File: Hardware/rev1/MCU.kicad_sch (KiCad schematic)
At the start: 5 parts, among them SW1 SW_Push, U1 STM32F103C8Tx, U4 W25Q128JVS

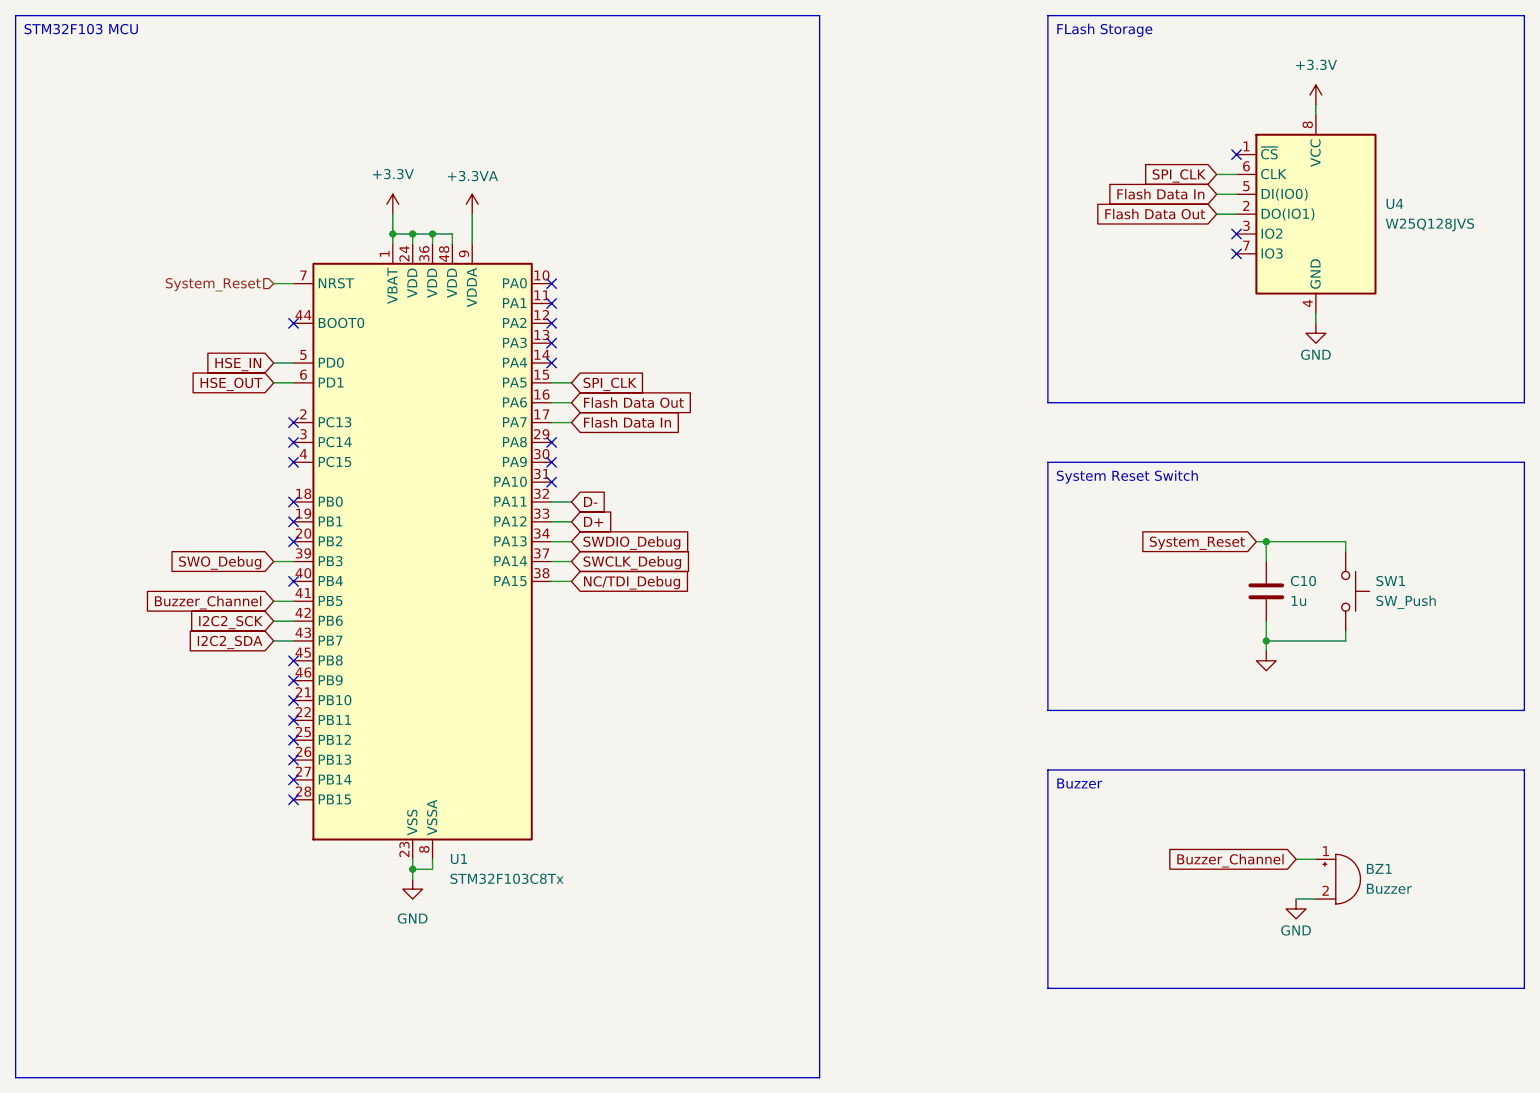
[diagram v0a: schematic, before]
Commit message: UUUUHHH
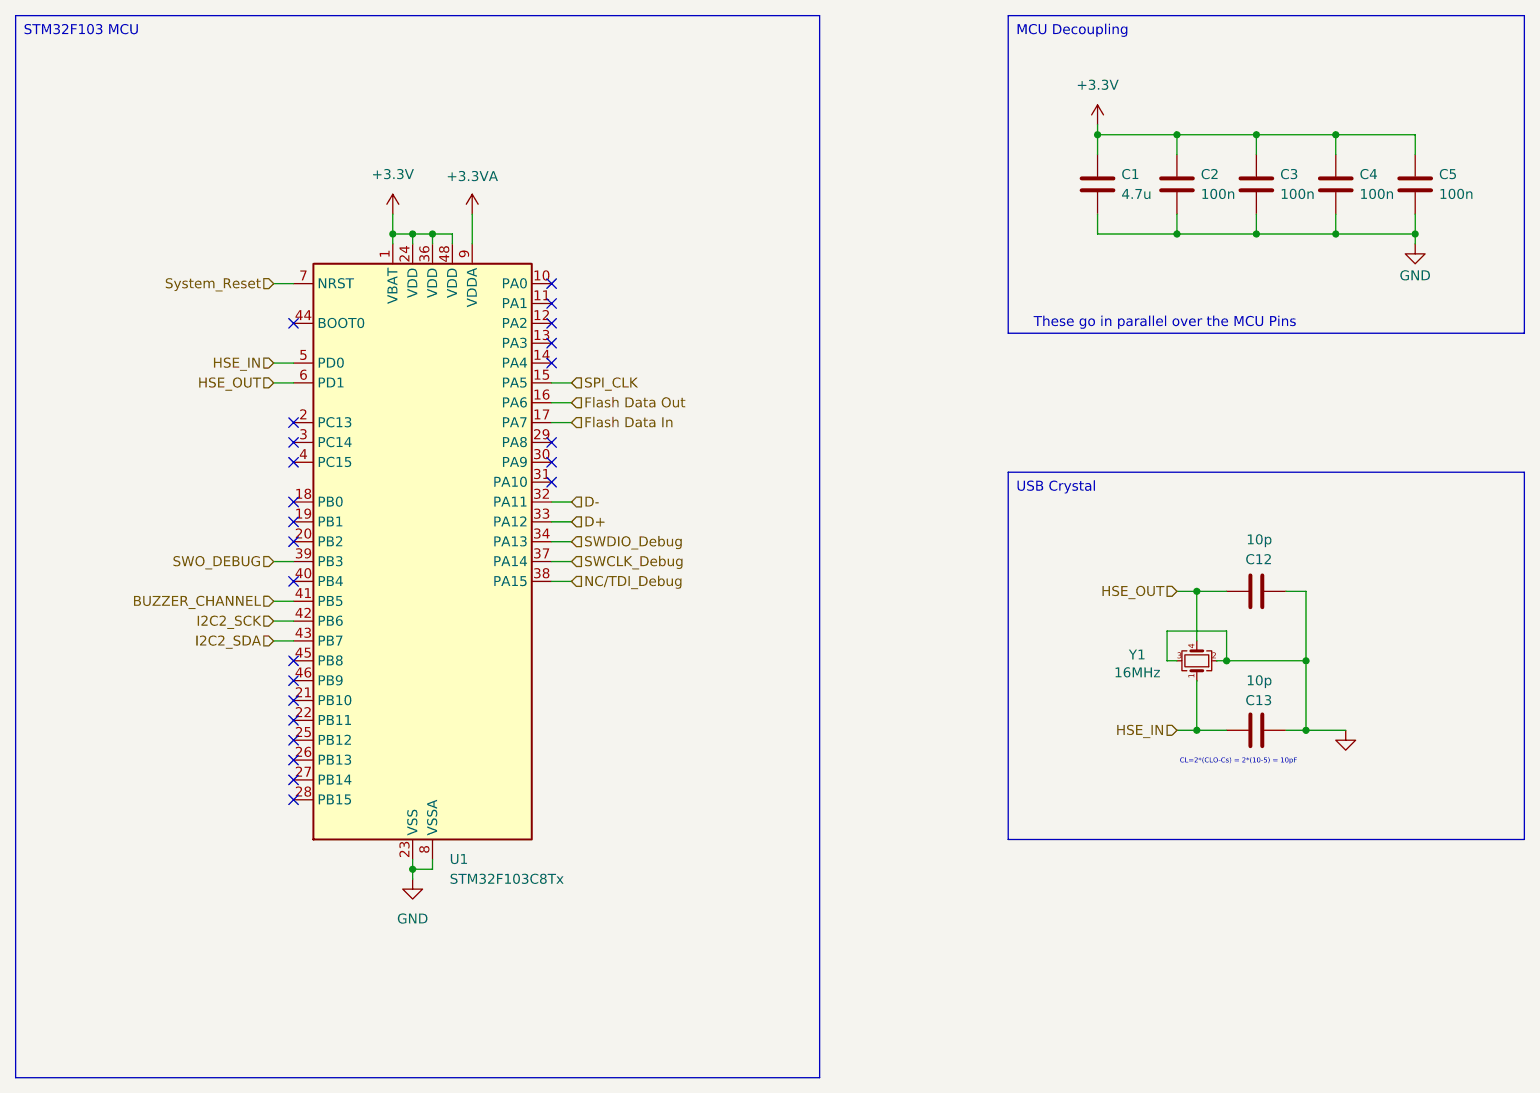
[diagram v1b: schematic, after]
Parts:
- removed BZ1: Buzzer, symbol Device:Buzzer
- removed C10: 1u, symbol Device:C
- removed SW1: SW_Push, symbol Switch:SW_Push
- removed U4: W25Q128JVS, Package_SO:SOIC-8_5.23x5.23mm_P1.27mm, symbol Memory_Flash:W25Q128JVS
- added C1: 4.7u, symbol Device:C
- added C12, C13: 10p, Capacitor_SMD:C_0402_1005Metric, symbol Device:C
- added C2, C3, C4, C5: 100n, symbol Device:C
- added Y1: 16MHz, Crystal:Crystal_SMD_3225-4Pin_3.2x2.5mm, symbol Device:Crystal_GND23_Small
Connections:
- net +3.3V: now also C1.1, C2.1, C3.1, C4.1, C5.1
- net GND: now also C1.2, C12.2, C13.2, C2.2, C3.2, C4.2, C5.2, Y1.2, Y1.3
- net HSE_IN: now also C13.1, Y1.1
- net HSE_OUT: now also C12.1, Y1.4
- net Buzzer_Channel renamed BUZZER_CHANNEL
- net SWO_Debug renamed SWO_DEBUG
- no-connect marks 27 -> 24
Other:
- note added: "CL=2*(CLO-Cs) = 2*(10-5) = 10pF"
- note added: "These go in parallel over the MCU Pins"
